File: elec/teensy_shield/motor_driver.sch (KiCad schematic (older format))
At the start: 0 parts

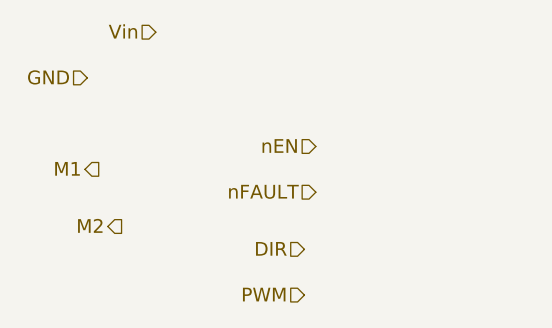
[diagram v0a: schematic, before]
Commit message: Completed new board schematics.
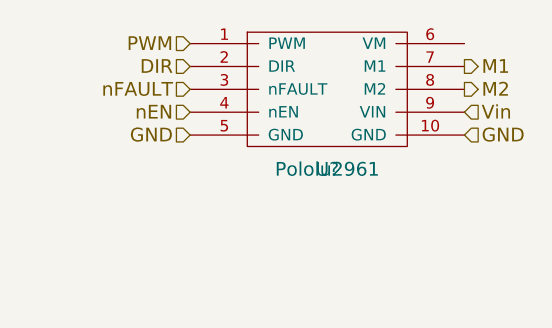
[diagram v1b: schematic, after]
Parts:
- added U?: Pololu2961, symbol Pololu2961
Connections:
- net DIR: now also U?.2 (DIR)
- net GND: now also U?.10 (GND), U?.5 (GND)
- net M1: now also U?.7 (M1)
- net M2: now also U?.8 (M2)
- net PWM: now also U?.1 (PWM)
- net Vin: now also U?.9 (VIN)
- net nEN: now also U?.4 (nEN)
- net nFAULT: now also U?.3 (nFAULT)
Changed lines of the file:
@@
 LIBS:contrib
 LIBS:valves
+LIBS:arduino_shieldsNCL
+LIBS:teensy
+LIBS:pololu
+LIBS:teensy_shield-cache
 EELAYER 24 0
 EELAYER END
 $Descr A4 11693 8268
 encoding utf-8
-Sheet 7 26
+Sheet 10 34
 Title ""
 Date ""
@@
 Comment4 ""
 $EndDescr
-Text HLabel 5100 2900 0    60   Input ~ 0
+Text HLabel 6450 3250 2    60   Input ~ 0
 Vin
-Text HLabel 4800 3100 0    60   Input ~ 0
+Text HLabel 5250 3350 0    60   Input ~ 0
 GND
-Text HLabel 4850 3500 0    60   Output ~ 0
+Text HLabel 6450 3050 2    60   Output ~ 0
 M1
-Text HLabel 4950 3750 0    60   Output ~ 0
+Text HLabel 6450 3150 2    60   Output ~ 0
 M2
-Text HLabel 5800 3400 0    60   Input ~ 0
+Text HLabel 5250 3250 0    60   Input ~ 0
 nEN
-Text HLabel 5800 3600 0    60   Input ~ 0
+Text HLabel 5250 3150 0    60   Input ~ 0
 nFAULT
-Text HLabel 5750 3850 0    60   Input ~ 0
+Text HLabel 5250 3050 0    60   Input ~ 0
 DIR
-Text HLabel 5750 4050 0    60   Input ~ 0
+Text HLabel 5250 2950 0    60   Input ~ 0
 PWM
+$Comp
+L Pololu2961 U?
+U 1 1 55E82F97
+P 5850 3150
+F 0 "U?" H 5850 2800 60  0000 C CNN
+F 1 "Pololu2961" H 5850 2800 60  0000 C CNN
+F 2 "" H 5850 2800 60  0000 C CNN
+F 3 "" H 5850 2800 60  0000 C CNN
+	1    5850 3150
+	1    0    0    -1
+$EndComp
+Text HLabel 6450 3350 2    60   Input ~ 0
+GND
 $EndSCHEMATC

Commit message: Elec ?
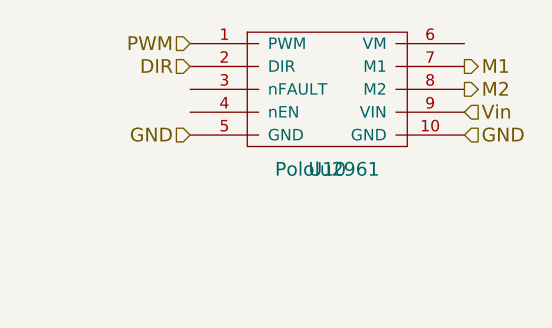
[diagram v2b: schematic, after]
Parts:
- gave numbers to parts that had none: 1
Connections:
- net nEN: no longer names the net of U13.4 (nEN)
- net nFAULT: no longer names the net of U13.3 (nFAULT)
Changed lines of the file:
@@
 $Descr A4 11693 8268
 encoding utf-8
-Sheet 10 34
+Sheet 24 34
 Title ""
 Date ""
@@
 Text HLabel 6450 3150 2    60   Output ~ 0
 M2
-Text HLabel 5250 3250 0    60   Input ~ 0
-nEN
-Text HLabel 5250 3150 0    60   Input ~ 0
-nFAULT
 Text HLabel 5250 3050 0    60   Input ~ 0
 DIR
@@
 PWM
 $Comp
-L Pololu2961 U?
+L Pololu2961 U13
 U 1 1 55E82F97
 P 5850 3150
-F 0 "U?" H 5850 2800 60  0000 C CNN
+AR Path="/55E6307C/55E6553A/55E82F97" Ref="U13"  Part="1"
+AR Path="/55E7381B/55E6553A/55E82F97" Ref="U4"  Part="1"
+AR Path="/55E7381C/55E6553A/55E82F97" Ref="U7"  Part="1"
+AR Path="/55E7381D/55E6553A/55E82F97" Ref="U10"  Part="1"
+F 0 "U10" H 5850 2800 60  0000 C CNN
 F 1 "Pololu2961" H 5850 2800 60  0000 C CNN
 F 2 "" H 5850 2800 60  0000 C CNN
